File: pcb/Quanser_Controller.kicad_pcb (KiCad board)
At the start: 2 copper layers, 115.6 x 61 mm, 24 parts, among them J1 Conn_02x08, J2 Connector Encoder, J3 Conn_01x10, J4 Conn_01x08, J5 Conn_01x08, J6 Conn_Coaxial, J6 Screw_Terminal_01x02, J7 Screw_Terminal_01x02, Q1 BC548, U1 LMD18200, U2 LS7366R, U3 74LVC1G04

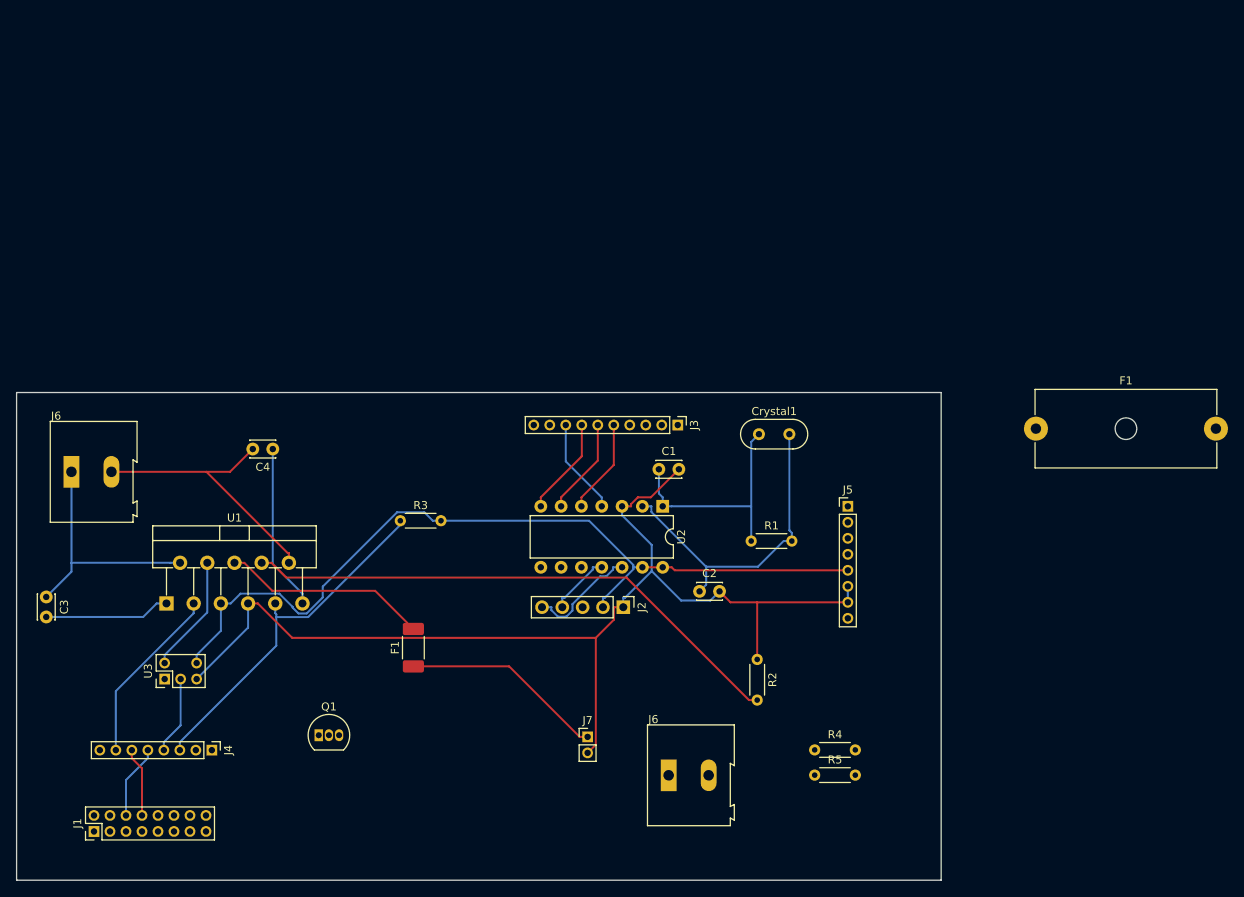
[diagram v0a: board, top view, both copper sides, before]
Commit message: update pcb
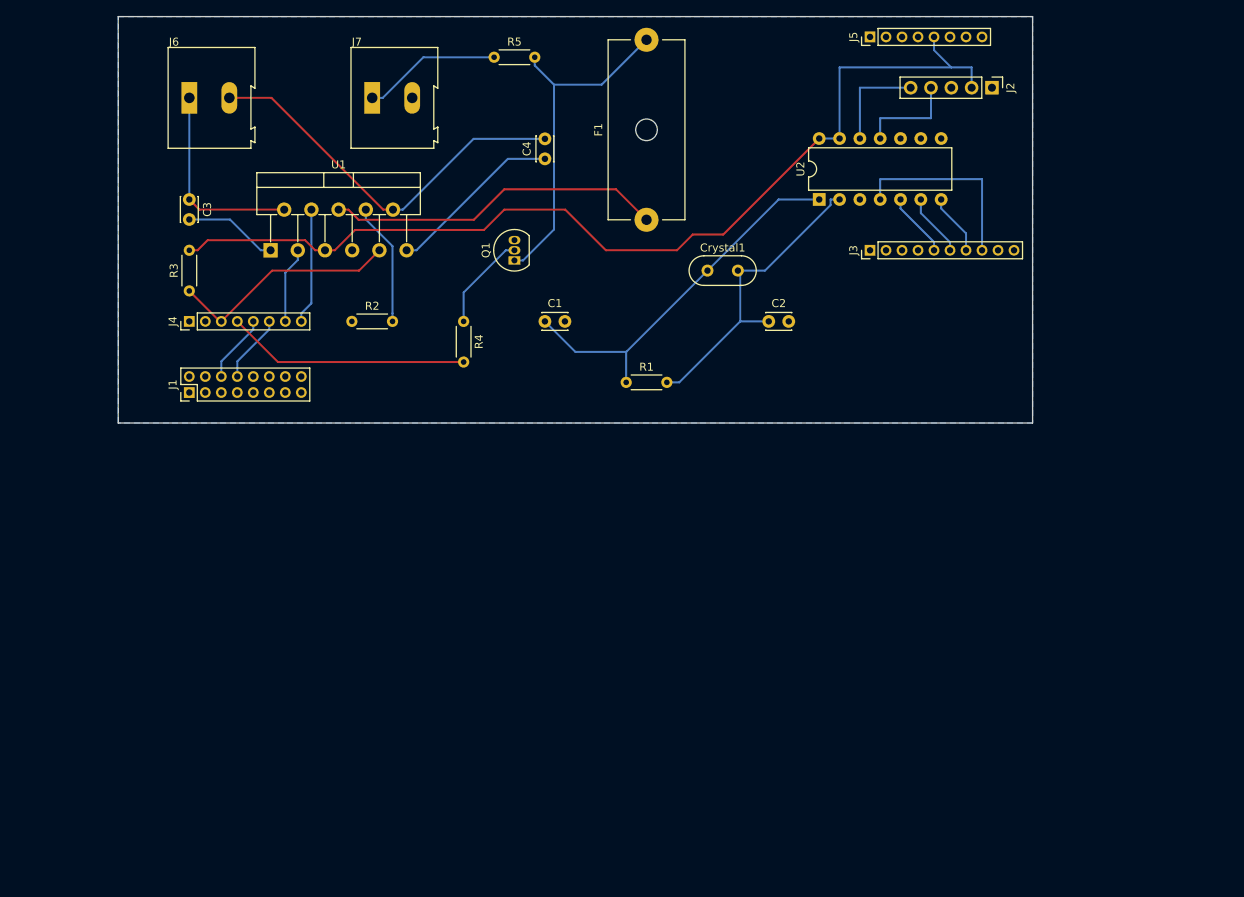
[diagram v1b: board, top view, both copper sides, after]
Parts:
- removed the F1 at (203.6, 102.3)
- removed the F1 at (125.8, 129.7)
- removed the J6 at (157.7, 145.6)
- removed the J6 at (83.1, 107.7)
- removed U3: 74LVC1G04, Connector_PinHeader_2.00mm:PinHeader_2x03_P2.00mm_Vertical
- added F1: 5A, Fuse:Fuseholder_Cylinder-5x20mm_Schurter_0031_8201_Horizontal_Open, F.Cu at (154.9, 76.2)
- added J6: Screw_Terminal_01x02, TerminalBlock:TerminalBlock_Altech_AK300-2_P5.00mm, F.Cu at (97.8, 61.0)
- J7: footprint Connector_PinHeader_2.00mm:PinHeader_1x02_P2.00mm_Vertical -> TerminalBlock:TerminalBlock_Altech_AK300-2_P5.00mm
- moved R5 98.3 mm to (135.9, 55.9)
- moved J7 84.3 mm to (120.7, 61.0)
- moved J2 79.6 mm to (198.1, 59.7)
- moved R4 69.2 mm to (132.1, 88.9), turned to 270 degrees
- moved R2 66.0 mm to (118.1, 88.9), turned to 0 degrees
- moved Q1 64.2 mm to (138.4, 81.3), turned to 90 degrees
- moved J5 58.7 mm to (182.9, 53.3), turned to 90 degrees
- moved J1 56.1 mm to (97.8, 97.8)
- moved J4 53.7 mm to (97.8, 88.9), turned to 90 degrees
- moved C3 52.8 mm to (97.8, 73.7)
- moved C4 49.7 mm to (142.2, 68.6), turned to 90 degrees
- moved U1 46.0 mm to (108.0, 80.0)
- moved U2 43.1 mm to (176.5, 73.7), turned to 90 degrees
- moved R3 39.0 mm to (97.8, 85.1), turned to 90 degrees
- moved C2 34.8 mm to (170.2, 88.9)
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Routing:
- net GND: track 139.3 -> 0.62 mm
- net Net-(R2-Pad2): track 69.0 -> 15.4 mm
- net Net-(F1-Pad1): track 0.00 -> 42.2 mm
- net DISABLE: track 0.00 -> 30.4 mm
- net +5V: track 104.6 -> 125.0 mm
- net Net-(C1-Pad1): track 29.7 -> 47.6 mm
- net Net-(F1-Pad2): track 25.8 -> 43.0 mm
- net TH_FLAG: track 44.2 -> 29.0 mm
- net Net-(U1-Pad4): track 14.7 -> 0.00 mm
- net BRAKE: track 0.00 -> 14.5 mm
- net Net-(C4-Pad2): track 34.6 -> 48.9 mm
- net PWM: track 22.4 -> 9.54 mm
- net Net-(Q1-Pad2): track 0.00 -> 12.2 mm
- net #SS: track 12.0 -> 24.1 mm
- net ENABLE: track 9.76 -> 0.00 mm
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- added copper zone on B.Cu, net GND
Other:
- board size 115.6 x 61 mm -> 114.3 x 50.8 mm
